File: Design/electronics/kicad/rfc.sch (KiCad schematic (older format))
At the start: 22 parts, among them IC1 L298, IC2 L298, J1 CONN_02X20, J2 CONN_01X03, J3 CONN_01X03, M1 Motor, M2 Motor, M3 Motor, M4 Motor, U1 HC-SR04, U2 HC-SR04, U3 HC-SR04, U4 HC-SR04

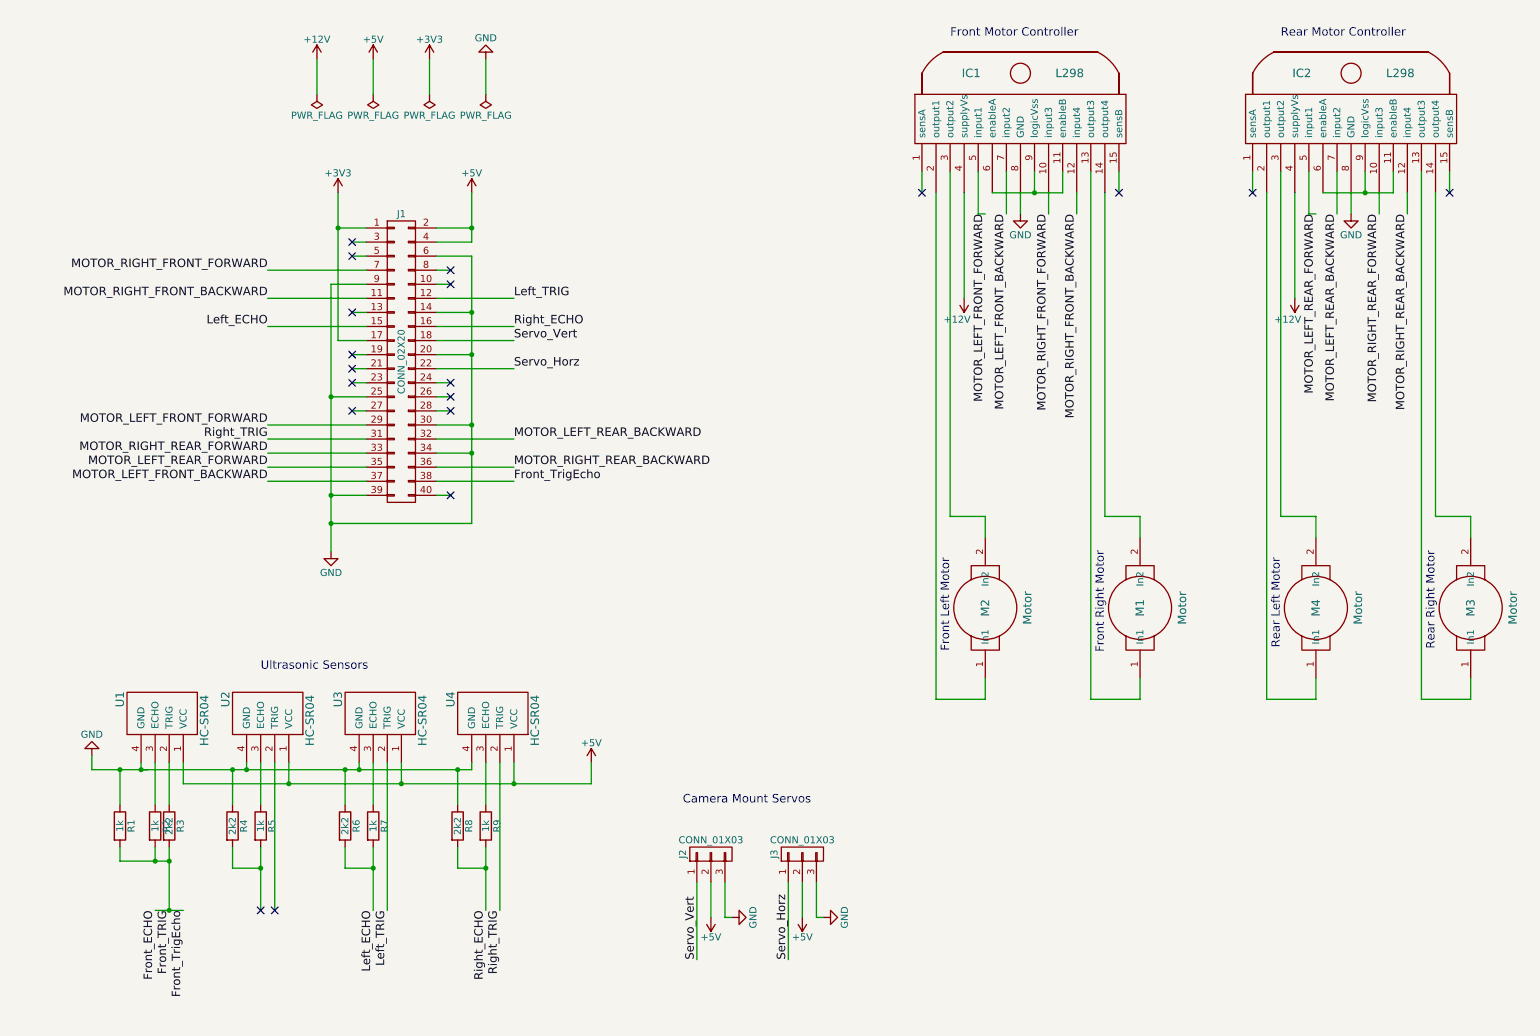
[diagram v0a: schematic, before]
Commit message: Updated schematic
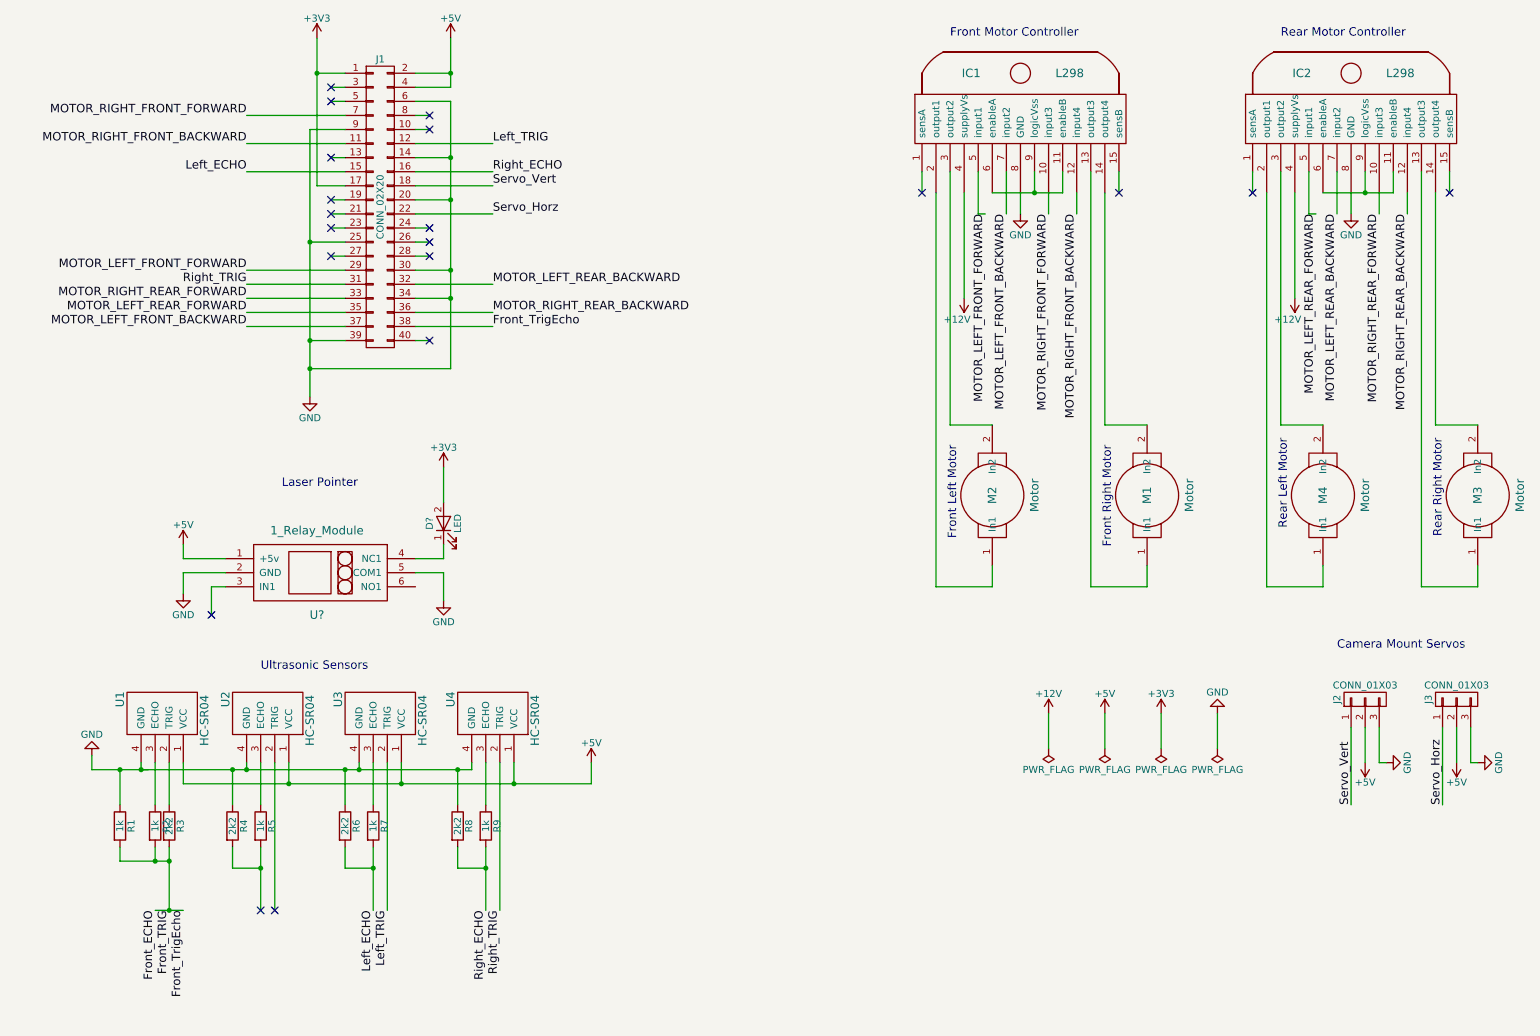
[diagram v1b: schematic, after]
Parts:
- added D?: LED, symbol LED
- added U?: 1_Relay_Module, symbol 1_Relay_Module
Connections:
- net +3V3: now also D?.2 (A)
- net +5V: now also U?.1 (+5v)
- net GND: now also U?.2 (GND), U?.5 (COM1)
- new net: D?.1 (K), U?.4 (NC1)
- no-connect marks 19 -> 20
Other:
- note added: "Laser Pointer"
- moved on the sheet: J1, J2, J3, M1, M2, M3, M4
